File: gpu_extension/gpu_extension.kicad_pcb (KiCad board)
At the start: 0 parts

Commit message: gpu and motherboard passes tests, now time for fpga
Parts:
- added C201: 14p, Capacitor_SMD:C_0603_1608Metric_Pad1.08x0.95mm_HandSolder, F.Cu at (78.0, 140.9)
- added C202: 14p, Capacitor_SMD:C_0603_1608Metric_Pad1.08x0.95mm_HandSolder, F.Cu at (75.5, 138.0)
- added C203: 100n, Capacitor_SMD:C_0603_1608Metric_Pad1.08x0.95mm_HandSolder, F.Cu at (60.6, 147.4)
- added C204: 100n, Capacitor_SMD:C_0603_1608Metric_Pad1.08x0.95mm_HandSolder, F.Cu at (64.7, 143.3)
- added C205: 100n, Capacitor_SMD:C_0603_1608Metric_Pad1.08x0.95mm_HandSolder, B.Cu at (70.6, 149.6)
- added C206: 100n, Capacitor_SMD:C_0603_1608Metric_Pad1.08x0.95mm_HandSolder, B.Cu at (68.4, 156.6)
- added C208: 1u, Capacitor_SMD:C_0603_1608Metric_Pad1.08x0.95mm_HandSolder, F.Cu at (64.1, 156.3)
- added C209: 100n, Capacitor_SMD:C_0603_1608Metric_Pad1.08x0.95mm_HandSolder, B.Cu at (68.8, 149.6)
- added C210: 100n, Capacitor_SMD:C_0603_1608Metric_Pad1.08x0.95mm_HandSolder, F.Cu at (60.0, 153.0)
- added C211: 100n, Capacitor_SMD:C_0603_1608Metric_Pad1.08x0.95mm_HandSolder, B.Cu at (66.7, 156.6)
- added C212: 100n, Capacitor_SMD:C_0603_1608Metric_Pad1.08x0.95mm_HandSolder, F.Cu at (66.4, 143.3)
- added C213: 100n, Capacitor_SMD:C_0603_1608Metric_Pad1.08x0.95mm_HandSolder, F.Cu at (62.3, 156.3)
- added C214: 1u, Capacitor_SMD:C_0603_1608Metric_Pad1.08x0.95mm_HandSolder, B.Cu at (64.0, 156.6)
- added C215: 100n, Capacitor_SMD:C_0603_1608Metric_Pad1.08x0.95mm_HandSolder, F.Cu at (58.4, 147.4)
- added C216: 100n, Capacitor_SMD:C_0603_1608Metric_Pad1.08x0.95mm_HandSolder, F.Cu at (58.5, 159.9)
- added C401: 100n, Capacitor_SMD:C_0603_1608Metric_Pad1.08x0.95mm_HandSolder, F.Cu at (48.0, 169.0)
- added C403: 100n, Capacitor_SMD:C_0603_1608Metric_Pad1.08x0.95mm_HandSolder, B.Cu at (70.0, 165.8)
- added C404: 1u, Capacitor_SMD:C_0603_1608Metric_Pad1.08x0.95mm_HandSolder, B.Cu at (65.2, 165.8)
- added J201: Conn_01x03_Male, Connector_PinHeader_2.54mm:PinHeader_1x03_P2.54mm_Vertical, F.Cu at (40.6, 164.0)
- added J301: DB15_Female_HighDensity, Connector_Dsub:DSUB-15_Female_Horizontal_P2.77x2.84mm_EdgePinOffset4.94mm_Housed_MountingHolesOffset7.48mm, F.Cu at (47.3, 130.6)
- added J302: HDMI_A, Connector_HDMI:HDMI_A_Molex_208658-1001_Horizontal, F.Cu at (40.0, 149.5)
- added J501: Conn_02x08_Odd_Even, Connector_PinHeader_2.54mm:PinHeader_2x08_P2.54mm_Horizontal, F.Cu at (75.8, 153.9)
- added R201: 1k, Resistor_SMD:R_0603_1608Metric_Pad0.98x0.95mm_HandSolder, F.Cu at (72.8, 140.9)
- added R301: 309, Resistor_SMD:R_0603_1608Metric_Pad0.98x0.95mm_HandSolder, F.Cu at (46.0, 137.0)
- added R302: 620, Resistor_SMD:R_0603_1608Metric_Pad0.98x0.95mm_HandSolder, F.Cu at (48.0, 137.0)
- added R303: 1240, Resistor_SMD:R_0603_1608Metric_Pad0.98x0.95mm_HandSolder, F.Cu at (50.0, 137.0)
- added R304: 309, Resistor_SMD:R_0603_1608Metric_Pad0.98x0.95mm_HandSolder, F.Cu at (61.0, 137.0)
- added R305: 620, Resistor_SMD:R_0603_1608Metric_Pad0.98x0.95mm_HandSolder, F.Cu at (59.0, 137.0)
- added R306: 1240, Resistor_SMD:R_0603_1608Metric_Pad0.98x0.95mm_HandSolder, F.Cu at (57.0, 137.0)
- added R307: 270, Resistor_SMD:R_0603_1608Metric_Pad0.98x0.95mm_HandSolder, F.Cu at (70.0, 136.9)
- added R308: 536, Resistor_SMD:R_0603_1608Metric_Pad0.98x0.95mm_HandSolder, F.Cu at (68.0, 136.9)
- added R309: 130, Resistor_SMD:R_0603_1608Metric_Pad0.98x0.95mm_HandSolder, F.Cu at (43.0, 136.1)
- added R310: 130, Resistor_SMD:R_0603_1608Metric_Pad0.98x0.95mm_HandSolder, F.Cu at (54.1, 136.1)
- added R311: 133, Resistor_SMD:R_0603_1608Metric_Pad0.98x0.95mm_HandSolder, F.Cu at (64.9, 136.0)
- added R315: 270, Resistor_SMD:R_0603_1608Metric_Pad0.98x0.95mm_HandSolder, F.Cu at (47.8, 157.4)
- added R316: 270, Resistor_SMD:R_0603_1608Metric_Pad0.98x0.95mm_HandSolder, F.Cu at (47.8, 153.7)
- added R317: 270, Resistor_SMD:R_0603_1608Metric_Pad0.98x0.95mm_HandSolder, F.Cu at (47.8, 150.1)
- added R318: 270, Resistor_SMD:R_0603_1608Metric_Pad0.98x0.95mm_HandSolder, F.Cu at (47.8, 146.5)
- added R319: 270, Resistor_SMD:R_0603_1608Metric_Pad0.98x0.95mm_HandSolder, F.Cu at (47.8, 155.5)
- added R320: 270, Resistor_SMD:R_0603_1608Metric_Pad0.98x0.95mm_HandSolder, F.Cu at (47.8, 151.9)
- added R321: 270, Resistor_SMD:R_0603_1608Metric_Pad0.98x0.95mm_HandSolder, F.Cu at (47.8, 148.3)
- added R322: 270, Resistor_SMD:R_0603_1608Metric_Pad0.98x0.95mm_HandSolder, F.Cu at (47.8, 144.7)
- added R401: 10k, Resistor_SMD:R_0603_1608Metric_Pad0.98x0.95mm_HandSolder, F.Cu at (57.6, 170.9)
- added R403: 10k, Resistor_SMD:R_0603_1608Metric_Pad0.98x0.95mm_HandSolder, B.Cu at (67.7, 170.8)
- added U1: SN74CBTLV3257PW, footprints:SOP63P599X175-16N, F.Cu at (54.6, 145.4)
- added U2: SN74CBTLV3257PW, footprints:SOP63P599X175-16N, F.Cu at (54.6, 156.2)
- added U3: APS6408L-3OBM-BA, footprints:BGA24C100P5X5_600X800X120, F.Cu at (67.7, 166.2)
- added U4: RP2040, footprints:QFN40P700X700X90-57N, F.Cu at (66.4, 149.7)
- added U401: W25Q128JVS, Package_SO:SOIC-8_5.23x5.23mm_P1.27mm, F.Cu at (54.6, 167.0)
- added Y201: ECS-120-8-36-CGN-TR, footprints:XTAL_ECS-120-8-36-CGN-TR, F.Cu at (75.5, 140.8)
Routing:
- net +5V: track 0.00 -> 101.8 mm, vias 0 -> 1
- net /RP2040/VGA.VSYNC: track 0.00 -> 63.0 mm, vias 0 -> 2
- net /RP2040/VGA.HSYNC: track 0.00 -> 62.9 mm, vias 0 -> 2
- net GND: track 0.00 -> 58.6 mm, vias 0 -> 50
- net +3V3: track 0.00 -> 52.9 mm, vias 0 -> 16
- net /RP2040/DEBUG.SWCLK: track 0.00 -> 36.0 mm, vias 0 -> 1
- net /RP2040/DEBUG.SWD: track 0.00 -> 35.7 mm, vias 0 -> 1
- net /RP2040/VGA.R0: track 0.00 -> 33.8 mm
- net /Memory/PSRAM.IO1: track 0.00 -> 33.6 mm
- net /Connector/BUS.CE#: track 0.00 -> 33.2 mm, vias 0 -> 1
- net /Connector/BUS.INT: track 0.00 -> 32.9 mm, vias 0 -> 1
- net /RP2040/VGA.R2: track 0.00 -> 32.5 mm, vias 0 -> 2
- net /RP2040/VGA.B1: track 0.00 -> 31.0 mm, vias 0 -> 2
- net /RP2040/VGA.B0: track 0.00 -> 30.9 mm, vias 0 -> 2
- net /RP2040/VGA.R1: track 0.00 -> 30.8 mm, vias 0 -> 2
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- added copper zone on In2.Cu, net +3V3
- added copper zone on In1.Cu, net GND
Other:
- board outline added: 46 x 49 mm
- copper layers 0 -> 4

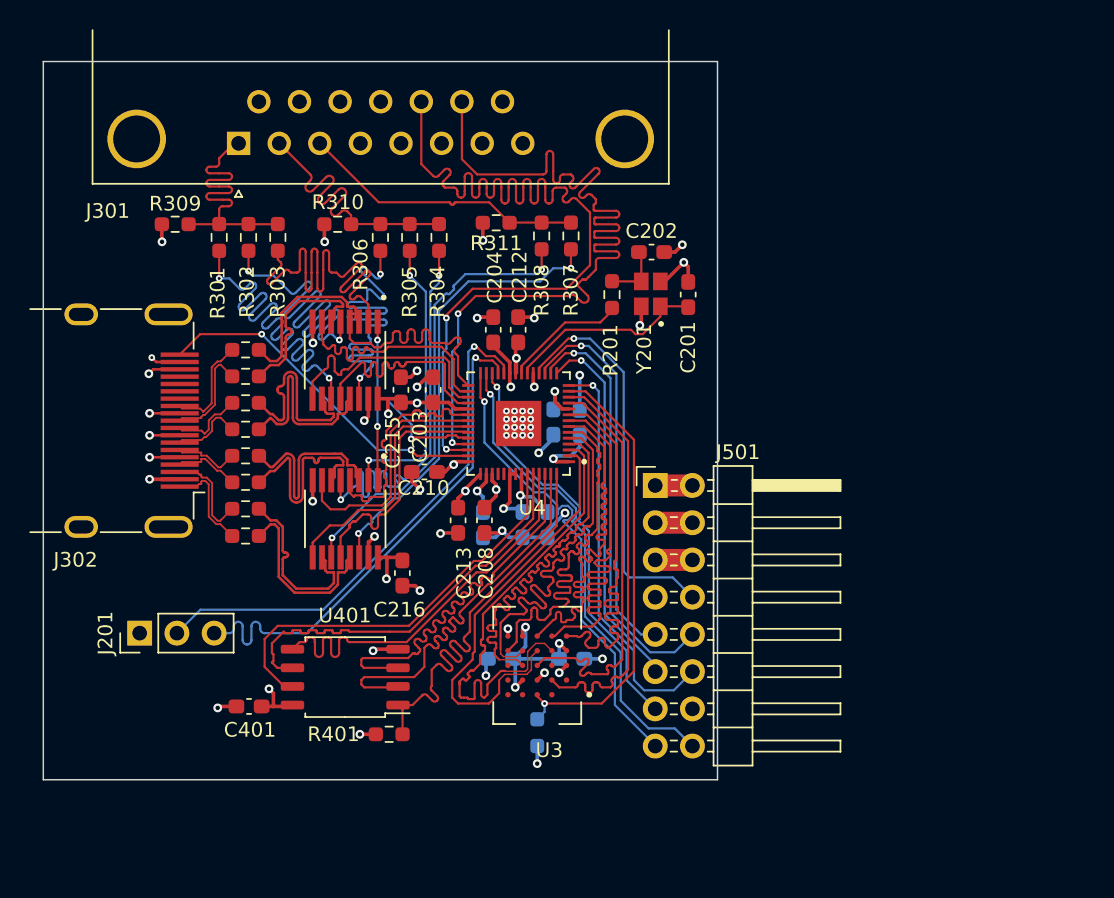
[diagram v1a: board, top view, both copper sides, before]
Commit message: fixes
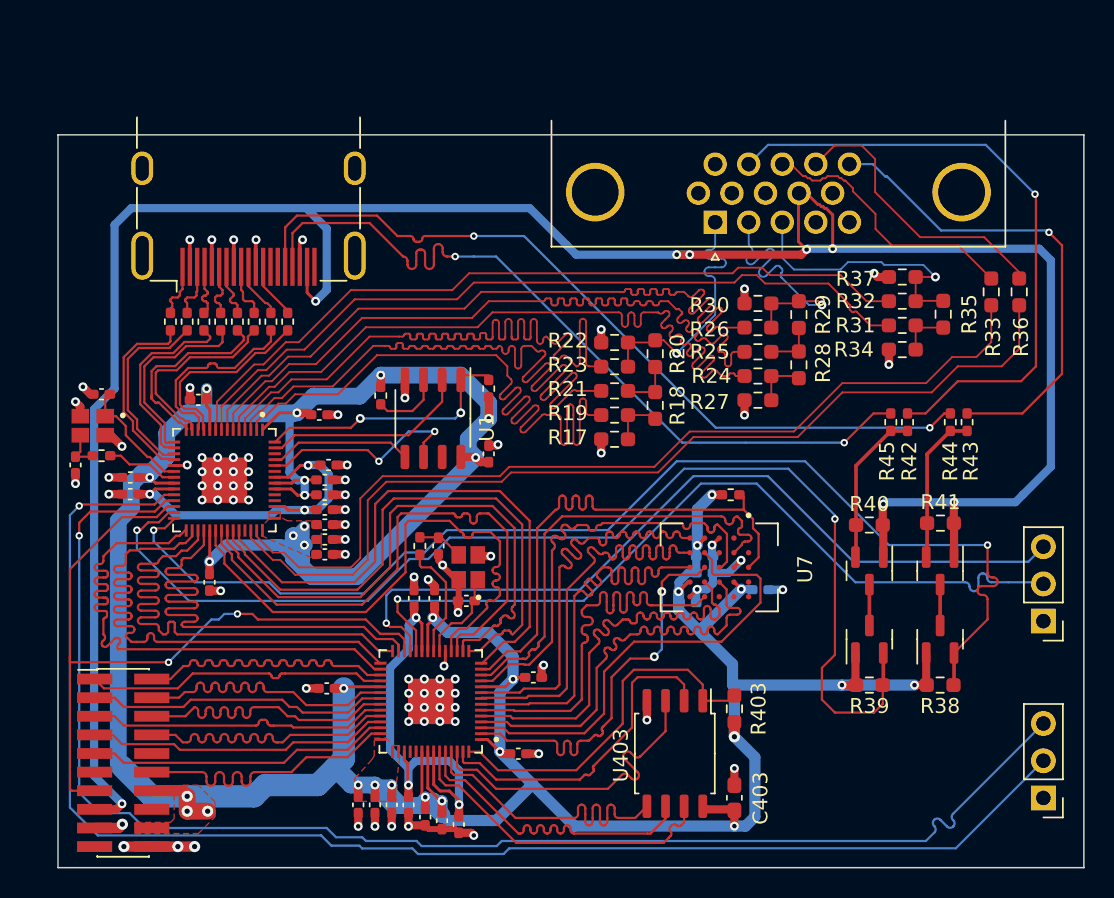
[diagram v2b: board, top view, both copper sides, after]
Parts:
- removed C401: 100n, Capacitor_SMD:C_0603_1608Metric_Pad1.08x0.95mm_HandSolder
- removed J301: DB15_Female_HighDensity, Connector_Dsub:DSUB-15_Female_Horizontal_P2.77x2.84mm_EdgePinOffset4.94mm_Housed_MountingHolesOffset7.48mm
- removed J501: Conn_02x08_Odd_Even, Connector_PinHeader_2.54mm:PinHeader_2x08_P2.54mm_Horizontal
- removed R301, R304: 309, Resistor_SMD:R_0603_1608Metric_Pad0.98x0.95mm_HandSolder
- removed R302, R305: 620, Resistor_SMD:R_0603_1608Metric_Pad0.98x0.95mm_HandSolder
- removed R303, R306: 1240, Resistor_SMD:R_0603_1608Metric_Pad0.98x0.95mm_HandSolder
- removed R307: 270, Resistor_SMD:R_0603_1608Metric_Pad0.98x0.95mm_HandSolder
- removed R308: 536, Resistor_SMD:R_0603_1608Metric_Pad0.98x0.95mm_HandSolder
- removed R309, R310: 130, Resistor_SMD:R_0603_1608Metric_Pad0.98x0.95mm_HandSolder
- removed R311: 133, Resistor_SMD:R_0603_1608Metric_Pad0.98x0.95mm_HandSolder
- removed R401: 10k, Resistor_SMD:R_0603_1608Metric_Pad0.98x0.95mm_HandSolder
- removed U2: SN74CBTLV3257PW, footprints:SOP63P599X175-16N
- removed U3: APS6408L-3OBM-BA, footprints:BGA24C100P5X5_600X800X120
- removed U401: W25Q128JVS, Package_SO:SOIC-8_5.23x5.23mm_P1.27mm
- added C207: 100n, Capacitor_SMD:C_0402_1005Metric_Pad0.74x0.62mm_HandSolder, F.Cu at (53.2, 156.6)
- added C217: 1u, Capacitor_SMD:C_0402_1005Metric_Pad0.74x0.62mm_HandSolder, F.Cu at (58.9, 175.7)
- added C218: 14p, Capacitor_SMD:C_0402_1005Metric_Pad0.74x0.62mm_HandSolder, F.Cu at (62.9, 161.8)
- added C219: 100n, Capacitor_SMD:C_0402_1005Metric_Pad0.74x0.62mm_HandSolder, F.Cu at (57.8, 175.7)
- added C220: 100n, Capacitor_SMD:C_0402_1005Metric_Pad0.74x0.62mm_HandSolder, F.Cu at (60.1, 176.5)
- added C221: 100n, Capacitor_SMD:C_0402_1005Metric_Pad0.74x0.62mm_HandSolder, F.Cu at (61.2, 176.8)
- added C222: 100n, Capacitor_SMD:C_0402_1005Metric_Pad0.74x0.62mm_HandSolder, F.Cu at (66.4, 172.2)
- added C223: 14p, Capacitor_SMD:C_0402_1005Metric_Pad0.74x0.62mm_HandSolder, F.Cu at (61.0, 158.1)
- added C224: 100n, Capacitor_SMD:C_0402_1005Metric_Pad0.74x0.62mm_HandSolder, F.Cu at (55.5, 175.7)
- added C225: 100n, Capacitor_SMD:C_0402_1005Metric_Pad0.74x0.62mm_HandSolder, F.Cu at (67.4, 167.0)
- added C226: 100n, Capacitor_SMD:C_0402_1005Metric_Pad0.74x0.62mm_HandSolder, F.Cu at (60.7, 161.6)
- added C227: 100n, Capacitor_SMD:C_0402_1005Metric_Pad0.74x0.62mm_HandSolder, F.Cu at (53.3, 167.8)
- added C228: 1u, Capacitor_SMD:C_0402_1005Metric_Pad0.74x0.62mm_HandSolder, F.Cu at (56.6, 175.7)
- added C405: 100n, Capacitor_SMD:C_0402_1005Metric_Pad0.74x0.62mm_HandSolder, B.Cu at (78.0, 161.9)
- added C406: 100n, Capacitor_SMD:C_0402_1005Metric_Pad0.74x0.62mm_HandSolder, B.Cu at (82.9, 161.0)
- added C407: 100n, Capacitor_SMD:C_0402_1005Metric_Pad0.74x0.62mm_HandSolder, B.Cu at (79.1, 158.8)
- added C408: 1u, Capacitor_SMD:C_0402_1005Metric_Pad0.74x0.62mm_HandSolder, B.Cu at (79.1, 159.9)
- added J1: Conn_02x10_Odd_Even, Connector_PinHeader_1.27mm:PinHeader_2x10_P1.27mm_Vertical_SMD, F.Cu at (39.5, 172.8)
- added J2: DB15_Female_HighDensity_MountingHoles, Connector_Dsub:DSUB-15-HD_Female_Horizontal_P2.29x1.98mm_EdgePinOffset3.03mm_Housed_MountingHolesOffset4.94mm, F.Cu at (79.8, 136.0)
- added J202: Conn_01x03_Male, Connector_PinHeader_2.54mm:PinHeader_1x03_P2.54mm_Vertical, F.Cu at (102.2, 163.2)
- added Q1: BS170F, Package_TO_SOT_SMD:SOT-23, F.Cu at (90.4, 164.4)
- added Q2: BS170F, Package_TO_SOT_SMD:SOT-23, F.Cu at (90.4, 159.7)
- added Q3: BS170F, Package_TO_SOT_SMD:SOT-23, F.Cu at (95.2, 164.4)
- added Q4: BS170F, Package_TO_SOT_SMD:SOT-23, F.Cu at (95.2, 159.7)
- added R17: 619, Resistor_SMD:R_0603_1608Metric_Pad0.98x0.95mm_HandSolder, F.Cu at (73.0, 150.8)
- added R18: 309, Resistor_SMD:R_0603_1608Metric_Pad0.98x0.95mm_HandSolder, F.Cu at (75.7, 148.5)
- added R19: 619, Resistor_SMD:R_0603_1608Metric_Pad0.98x0.95mm_HandSolder, F.Cu at (73.0, 149.1)
- added R20: 309, Resistor_SMD:R_0603_1608Metric_Pad0.98x0.95mm_HandSolder, F.Cu at (75.7, 144.9)
- added R202: 1k, Resistor_SMD:R_0402_1005Metric_Pad0.72x0.64mm_HandSolder, F.Cu at (59.7, 158.1)
- added R21: 619, Resistor_SMD:R_0603_1608Metric_Pad0.98x0.95mm_HandSolder, F.Cu at (73.0, 147.5)
- added R22: 97.6, Resistor_SMD:R_0603_1608Metric_Pad0.98x0.95mm_HandSolder, F.Cu at (73.0, 144.2)
- added R23: 619, Resistor_SMD:R_0603_1608Metric_Pad0.98x0.95mm_HandSolder, F.Cu at (73.0, 145.8)
- added R24: 619, Resistor_SMD:R_0603_1608Metric_Pad0.98x0.95mm_HandSolder, F.Cu at (82.8, 146.5)
- added R25: 619, Resistor_SMD:R_0603_1608Metric_Pad0.98x0.95mm_HandSolder, F.Cu at (82.8, 144.8)
- added R26: 619, Resistor_SMD:R_0603_1608Metric_Pad0.98x0.95mm_HandSolder, F.Cu at (82.8, 143.2)
- added R27: 619, Resistor_SMD:R_0603_1608Metric_Pad0.98x0.95mm_HandSolder, F.Cu at (82.8, 148.1)
- added R28: 309, Resistor_SMD:R_0603_1608Metric_Pad0.98x0.95mm_HandSolder, F.Cu at (85.6, 145.7)
- added R29: 309, Resistor_SMD:R_0603_1608Metric_Pad0.98x0.95mm_HandSolder, F.Cu at (85.6, 142.3)
- added R30: 97.6, Resistor_SMD:R_0603_1608Metric_Pad0.98x0.95mm_HandSolder, F.Cu at (82.8, 141.5)
- added R31: 536, Resistor_SMD:R_0603_1608Metric_Pad0.98x0.95mm_HandSolder, F.Cu at (92.6, 143.0)
- added R32: 536, Resistor_SMD:R_0603_1608Metric_Pad0.98x0.95mm_HandSolder, F.Cu at (92.6, 141.4)
- added R33: 47, Resistor_SMD:R_0603_1608Metric_Pad0.98x0.95mm_HandSolder, F.Cu at (98.7, 140.7)
- added R34: 536, Resistor_SMD:R_0603_1608Metric_Pad0.98x0.95mm_HandSolder, F.Cu at (92.6, 144.7)
- added R35: 267, Resistor_SMD:R_0603_1608Metric_Pad0.98x0.95mm_HandSolder, F.Cu at (95.4, 142.2)
- added R36: 47, Resistor_SMD:R_0603_1608Metric_Pad0.98x0.95mm_HandSolder, F.Cu at (100.6, 140.7)
- added R37: 105, Resistor_SMD:R_0603_1608Metric_Pad0.98x0.95mm_HandSolder, F.Cu at (92.6, 139.7)
- added R38: 10k, Resistor_SMD:R_0603_1608Metric_Pad0.98x0.95mm_HandSolder, F.Cu at (95.2, 167.5)
- added R39: 10k, Resistor_SMD:R_0603_1608Metric_Pad0.98x0.95mm_HandSolder, F.Cu at (90.4, 167.5)
- added R40: 10k, Resistor_SMD:R_0603_1608Metric_Pad0.98x0.95mm_HandSolder, F.Cu at (90.4, 156.6)
- added R404: 10k, Resistor_SMD:R_0402_1005Metric_Pad0.72x0.64mm_HandSolder, F.Cu at (57.0, 147.8)
- added R405: 10k, Resistor_SMD:R_0402_1005Metric_Pad0.72x0.64mm_HandSolder, F.Cu at (80.9, 154.6)
- added R406: 10k, Resistor_SMD:R_0402_1005Metric_Pad0.72x0.64mm_HandSolder, F.Cu at (64.4, 147.3)
- added R41: 10k, Resistor_SMD:R_0603_1608Metric_Pad0.98x0.95mm_HandSolder, F.Cu at (95.2, 156.5)
- added R42: 0, Resistor_SMD:R_0402_1005Metric_Pad0.72x0.64mm_HandSolder, F.Cu at (93.0, 149.6)
- added R43: 0, Resistor_SMD:R_0402_1005Metric_Pad0.72x0.64mm_HandSolder, F.Cu at (97.0, 149.6)
- added R44: 0, Resistor_SMD:R_0402_1005Metric_Pad0.72x0.64mm_HandSolder, F.Cu at (95.9, 149.6)
- added R45: 0, Resistor_SMD:R_0402_1005Metric_Pad0.72x0.64mm_HandSolder, F.Cu at (91.8, 149.6)
- added U403: W25Q128JVS, Package_SO:SOIC-8_5.23x5.23mm_P1.27mm, F.Cu at (77.1, 172.2)
- added U6: RP2040, footprints:QFN40P700X700X90-57N, F.Cu at (60.4, 168.7)
- added U7: APS6408L-3OBM-BA, footprints:BGA24C100P5X5_600X800X120, F.Cu at (80.1, 159.5)
- added Y202: ECS-120-8-36-CGN-TR, footprints:XTAL_ECS-120-8-36-CGN-TR, F.Cu at (63.0, 159.5)
- C201, C202, C203, C204, C208, C210, C212, C213, C215, C216: footprint Capacitor_SMD:C_0603_1608Metric_Pad1.08x0.95mm_HandSolder -> Capacitor_SMD:C_0402_1005Metric_Pad0.74x0.62mm_HandSolder
- C205, C206, C209, C211, C214: footprint Capacitor_SMD:C_0603_1608Metric_Pad1.08x0.95mm_HandSolder -> Capacitor_SMD:C_0402_1005Metric_Pad0.74x0.62mm_HandSolder; moved to F.Cu
- C403, R403: moved to F.Cu
- C404: value 1u -> 100n; footprint Capacitor_SMD:C_0603_1608Metric_Pad1.08x0.95mm_HandSolder -> Capacitor_SMD:C_0402_1005Metric_Pad0.74x0.62mm_HandSolder; moved to F.Cu
- J302: value HDMI_A -> NOT_HDMI_A
- R201, R315, R316, R317, R318, R319, R320, R321, R322: footprint Resistor_SMD:R_0603_1608Metric_Pad0.98x0.95mm_HandSolder -> Resistor_SMD:R_0402_1005Metric_Pad0.72x0.64mm_HandSolder
- U1: value SN74CBTLV3257PW -> GD25D05CT; footprint footprints:SOP63P599X175-16N -> Package_SO:SOP-8_3.9x4.9mm_P1.27mm
- moved J201 62.7 mm to (102.2, 175.2), turned to 180 degrees
- moved C202 41.9 mm to (36.2, 152.5), turned to -90 degrees
- moved C201 40.6 mm to (38.0, 147.7), turned to 180 degrees
- moved Y201 39.1 mm to (37.4, 149.8), turned to 180 degrees
- moved R201 36.5 mm to (38.0, 151.9), turned to 0 degrees
- moved C206 28.5 mm to (39.9, 154.5), turned to 180 degrees
- moved C212 27.2 mm to (45.3, 160.5), turned to -90 degrees
- moved U4 20.4 mm to (46.4, 153.6), turned to -90 degrees
- moved C210 20.1 mm to (39.9, 153.4)
- moved C205 17.8 mm to (53.2, 153.5), turned to 0 degrees
- moved C216 17.6 mm to (62.3, 177.1)
- moved C209 16.4 mm to (53.2, 154.6), turned to 0 degrees
- moved C203 16.0 mm to (44.6, 148.1), turned to 180 degrees
- moved J302 15.9 mm to (48.0, 135.7), turned to 90 degrees
- moved C211 15.8 mm to (52.8, 149.1), turned to 0 degrees
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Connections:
- net /RP2040/DEBUG.SWCLK renamed /DEBUG.SWCLK
- net /RP2040/DEBUG.SWD renamed /DEBUG.SWD
- net /RP2040/OSC_IN renamed /OSC_IN
- net /RP2040/OSC_OUT renamed /OSC_OUT
- net /Video Output/TDMS_CK+ renamed Net-(J302-CK+)
- net /Video Output/TDMS_CK- renamed Net-(J302-CK-)
- net /Video Output/TDMS_D0+ renamed Net-(J302-D0+)
- net /Video Output/TDMS_D0- renamed Net-(J302-D0-)
- net /Video Output/TDMS_D1+ renamed Net-(J302-D1+)
- net /Video Output/TDMS_D1- renamed Net-(J302-D1-)
- net /Video Output/TDMS_D2+ renamed Net-(J302-D2+)
- net /Video Output/TDMS_D2- renamed Net-(J302-D2-)
- C215 pad 1: +3V3 -> +1V1_RENDER
- C216 pad 1: +3V3 -> +1V1_RENDER
- J302 pad 15: unconnected-(J302-SCL) -> Net-(J302-SCL)
- J302 pad 16: unconnected-(J302-SDA) -> Net-(J302-SDA)
- J302 pad 19: /RP2040/DVI.HPD -> unconnected-(J302-HPD)
- R315 pad 1: /RP2040/DVI.D2+ -> /DVI connector/DVI.D2+
- R316 pad 1: /RP2040/DVI.D1+ -> /DVI connector/DVI.D1+
- R317 pad 1: /RP2040/DVI.D0+ -> /DVI connector/DVI.D0+
- R318 pad 1: /RP2040/DVI.CK+ -> /DVI connector/DVI.CK+
- R319 pad 1: /RP2040/DVI.D2- -> /DVI connector/DVI.D2-
- R320 pad 1: /RP2040/DVI.D1- -> /DVI connector/DVI.D1-
- R321 pad 1: /RP2040/DVI.D0- -> /DVI connector/DVI.D0-
- R322 pad 1: /RP2040/DVI.CK- -> /DVI connector/DVI.CK-
- R403 pad 2: /Memory/PSRAM.CE# -> /Render Engine/Memory Render Engine/FLASH_ENGINE.CS#
- U1 pad 1: /RP2040/SELECT_OUTPUT -> /Memory/FLASH.CS#
- U1 pad 2: /RP2040/VGA.R0 -> /Memory/FLASH.IO1
- U1 pad 3: /RP2040/DVI.CK- -> Net-(U1-~{WP})
- U1 pad 4: /RP2040/IO0 -> GND
- U1 pad 5: /RP2040/VGA.R1 -> /Memory/FLASH.IO0
- U1 pad 6: /RP2040/DVI.CK+ -> /Memory/FLASH.CLK
- U1 pad 7: /RP2040/IO1 -> unconnected-(U1-NC)
- U1 pad 8: GND -> +3V3
- U4 pad 11: /Memory/PSRAM.RWDS -> /DVI connector/DVI.CK-
- U4 pad 12: /Memory/PSRAM.CLK -> /DVI connector/DVI.CK+
- U4 pad 13: /Memory/PSRAM.CE# -> /DVI connector/DVI.D0-
- U4 pad 14: /Connector/BUS.CLK -> /DVI connector/DVI.D0+
- U4 pad 15: /Connector/BUS.D0 -> /DVI connector/DVI.D1-
- U4 pad 16: /Connector/BUS.D1 -> /DVI connector/DVI.D1+
- U4 pad 17: /Connector/BUS.D2 -> /DVI connector/DVI.D2-
- U4 pad 18: /Connector/BUS.D3 -> /DVI connector/DVI.D2+
- U4 pad 2: /Memory/PSRAM.IO0 -> /DVI connector/VGA.R0
- U4 pad 26: /Connector/BUS.RE# -> /Render Engine/BUS connector/BUS.RE#
- U4 pad 27: /Connector/BUS.CE# -> /DVI connector/MCU_I2C.DATA
- U4 pad 28: /Connector/BUS.INT -> /DVI connector/MCU_I2C.CLOCK
- U4 pad 29: /RP2040/IO0 -> /Render Engine/OUT_BUS.CLK
- U4 pad 3: /Memory/PSRAM.IO1 -> /DVI connector/VGA.R1
- U4 pad 30: /RP2040/IO1 -> /Render Engine/OUT_BUS.D7
- U4 pad 31: /RP2040/IO2 -> /Render Engine/OUT_BUS.D6
- U4 pad 32: /RP2040/IO3 -> /Render Engine/OUT_BUS.D5
- U4 pad 34: /RP2040/IO4 -> /Render Engine/OUT_BUS.D4
- U4 pad 35: /RP2040/IO5 -> /Render Engine/OUT_BUS.D3
- U4 pad 36: /RP2040/IO6 -> /Render Engine/OUT_BUS.D2
- U4 pad 37: /RP2040/IO7 -> /Render Engine/OUT_BUS.D1
- U4 pad 38: /RP2040/SELECT_OUTPUT -> /Render Engine/OUT_BUS.D0
- U4 pad 39: /RP2040/VGA.VSYNC -> unconnected-(U4-GPIO27/ADC1)
- U4 pad 4: /Memory/PSRAM.IO2 -> /DVI connector/VGA.R2
- U4 pad 40: /RP2040/VGA.HSYNC -> /DVI connector/VGA.VSYNC
- U4 pad 41: /RP2040/DVI.HPD -> /DVI connector/VGA.HSYNC
- U4 pad 5: /Memory/PSRAM.IO3 -> /DVI connector/VGA.G0
- U4 pad 51: /Memory/FLASH.IO3 -> unconnected-(U4-QSPI_SD3)
- U4 pad 54: /Memory/FLASH.IO2 -> unconnected-(U4-QSPI_SD2)
- U4 pad 6: /Memory/PSRAM.IO4 -> /DVI connector/VGA.G1
- U4 pad 7: /Memory/PSRAM.IO5 -> /DVI connector/VGA.G2
- U4 pad 8: /Memory/PSRAM.IO6 -> /DVI connector/VGA.B0
- U4 pad 9: /Memory/PSRAM.IO7 -> /DVI connector/VGA.B1
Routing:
- net +3V3: track 52.9 -> 306.4 mm, vias 16 -> 32
- net /DVI connector/MCU_I2C.DATA: track 0.00 -> 79.6 mm, vias 0 -> 2
- net /DVI connector/MCU_I2C.CLOCK: track 0.00 -> 79.4 mm, vias 0 -> 2
- net /DVI connector/VGA.VSYNC: track 0.00 -> 65.7 mm
- net /RP2040/VGA.VSYNC: track 63.0 -> 0.00 mm, vias 2 -> 0
- net /RP2040/VGA.HSYNC: track 62.9 -> 0.00 mm, vias 2 -> 0
- net /DVI connector/VGA.HSYNC: track 0.00 -> 62.7 mm
- net /DEBUG.SWD: track 35.7 -> 97.9 mm
- net /DEBUG.SWCLK: track 36.0 -> 98.0 mm
- net +5V: track 101.8 -> 163.1 mm, vias 1 -> 8
- net /Render Engine/DEBUG.SWD: track 0.00 -> 56.0 mm, vias 0 -> 1
- net /Render Engine/DEBUG.SWCLK: track 0.00 -> 55.9 mm, vias 0 -> 1
- net Net-(J302-SCL): track 0.00 -> 55.2 mm, vias 0 -> 2
- net Net-(J302-SDA): track 0.00 -> 55.1 mm, vias 0 -> 2
- net /DVI connector/VGA.B1: track 0.00 -> 52.5 mm
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- added copper zone on F.Cu, net +3V3
- added copper zone on In2.Cu, net GND
- removed copper zone on In2.Cu, net +3V3
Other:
- board size 46 x 49 mm -> 70 x 50 mm
